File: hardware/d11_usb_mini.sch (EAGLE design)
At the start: 20 parts, among them IC1 MIC5504-3.3, IC2 ATSAMD11C, J5 SIO, J6 SCK, J7 RST, J8 GND, X1 MINI-USB-32005-201

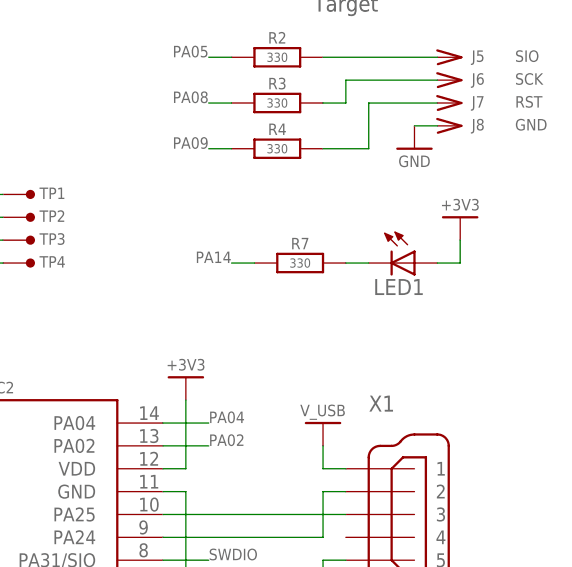
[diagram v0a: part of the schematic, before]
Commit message: Minor hardware changes + bootloader mode
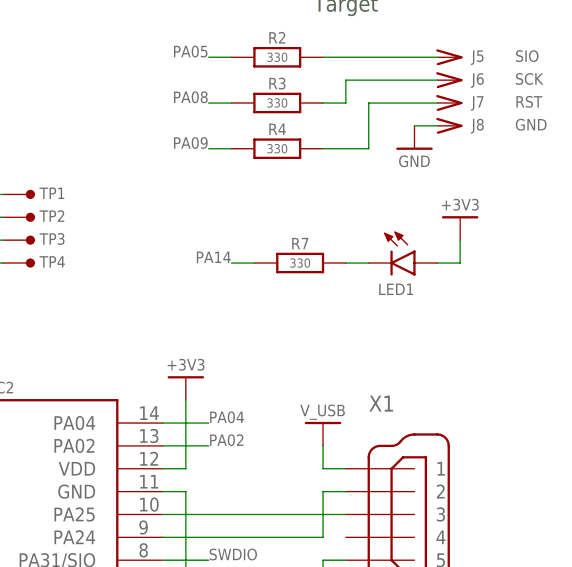
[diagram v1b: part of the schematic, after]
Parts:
- LED1: device led:LEDCHIPLED_0603 -> ataradov_led:LED_SMDLED_0603
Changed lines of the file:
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@@
 <part name="TP4" library="ataradov_misc" deviceset="TEST-POINT" device="-1.27MM"/>
 <part name="P_5" library="ataradov_pwr" deviceset="+3V3" device=""/>
-<part name="LED1" library="led" deviceset="LED" device="CHIPLED_0603"/>
+<part name="LED1" library="ataradov_led" deviceset="LED_SMD" device="LED_0603"/>
 </parts>
 <sheets>
@@
 <segment>
 <pinref part="R7" gate="G$1" pin="2"/>
+<wire x1="78.74" y1="78.74" x2="81.28" y2="78.74" width="0.1524" layer="91"/>
 <pinref part="LED1" gate="G$1" pin="C"/>
-<wire x1="78.74" y1="78.74" x2="81.28" y2="78.74" width="0.1524" layer="91"/>
-</segment>
-</net>
+</segment>
+</net>
